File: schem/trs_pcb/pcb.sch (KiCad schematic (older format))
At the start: 10 parts, among them J101 2x3 female, J102 2x3 female, U101 74HCT245, U102 74HC165, U103 74HC595, U104 74HC595

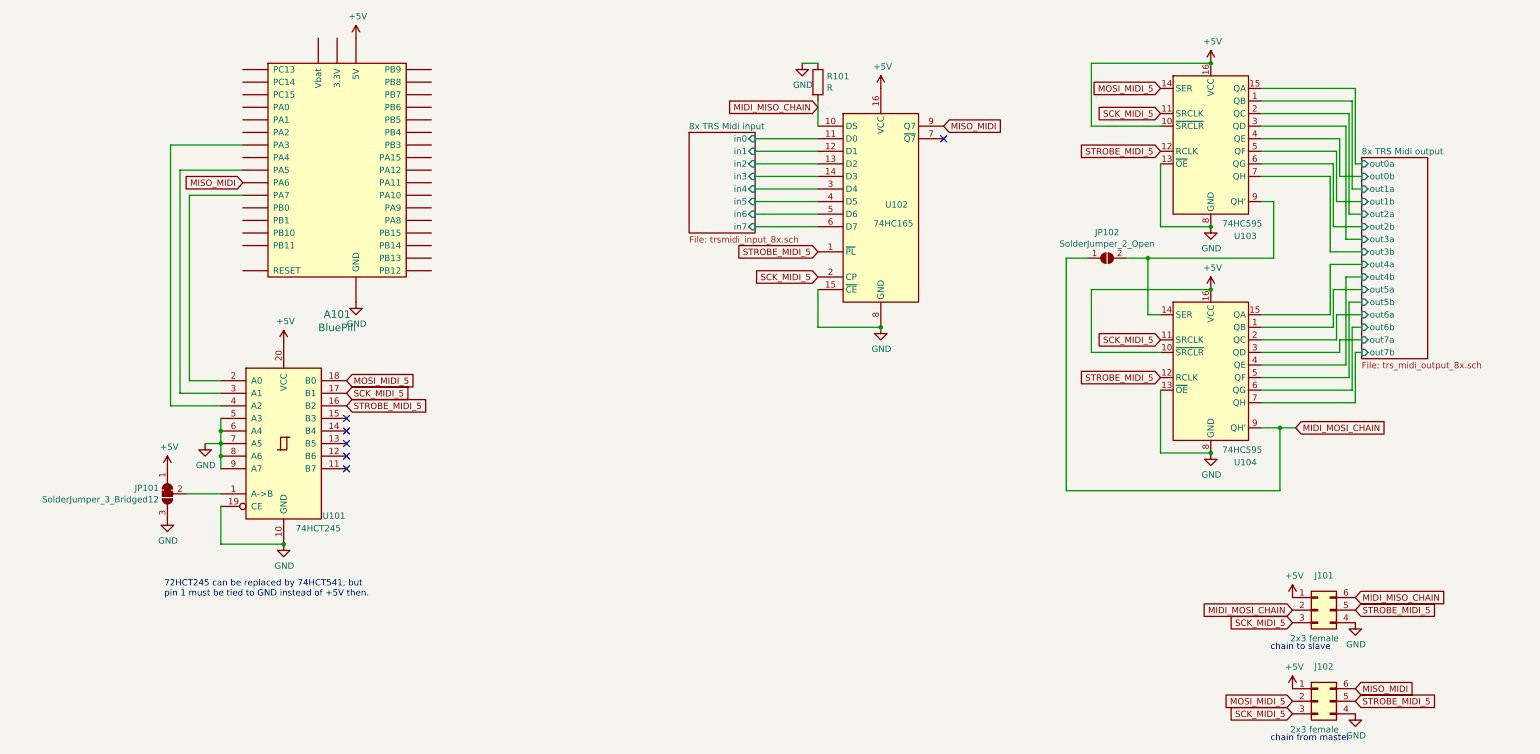
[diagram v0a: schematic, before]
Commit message: Come layout considerations
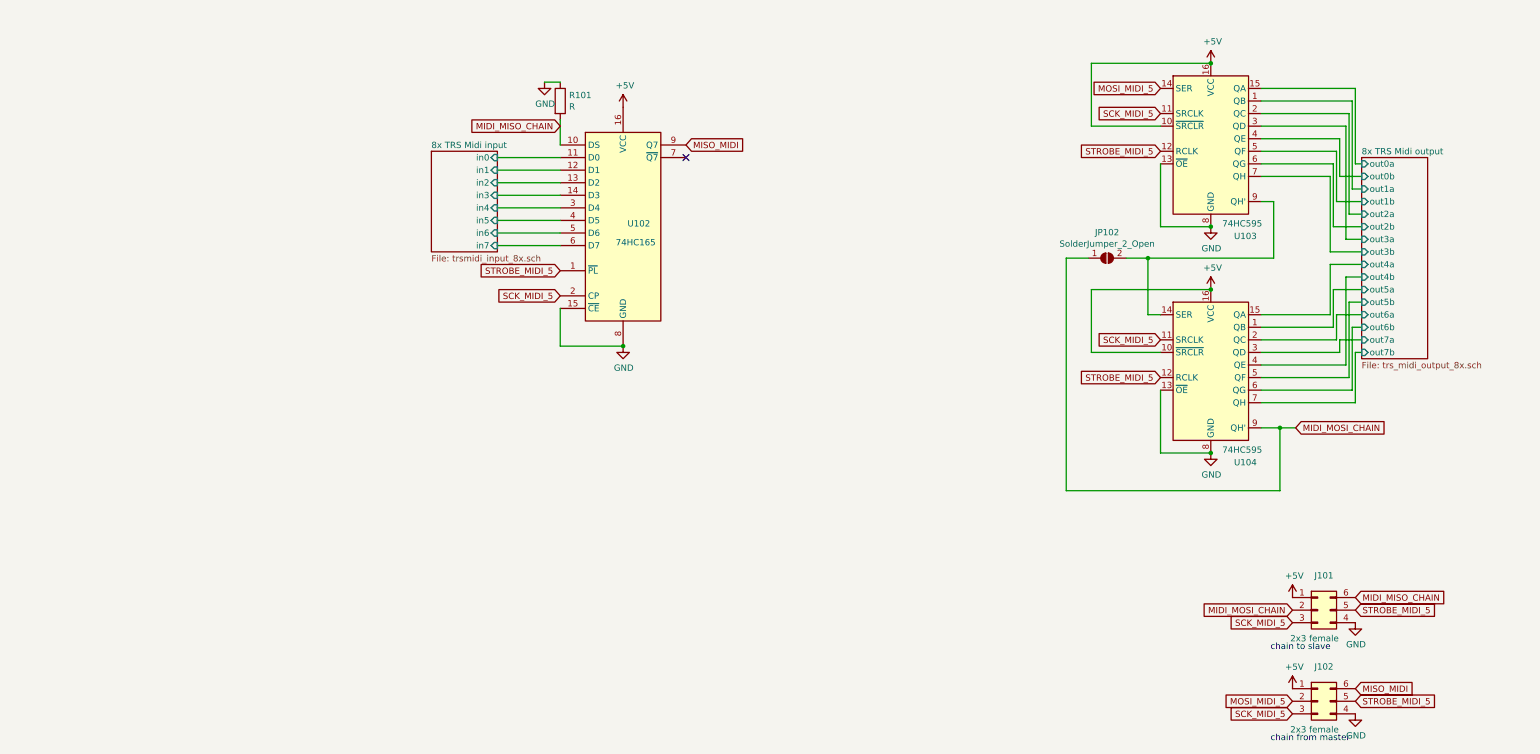
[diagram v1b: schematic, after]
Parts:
- removed A101: BluePill, footprints:BLUEPILL, symbol bluepill:BluePill
- removed JP101: SolderJumper_3_Bridged12, Jumper:SolderJumper-3_P2.0mm_Open_TrianglePad1.0x1.5mm, symbol Jumper:SolderJumper_3_Bridged12
- removed U101: 74HCT245, Package_DIP:DIP-20_W7.62mm, symbol 74xx:74HC245
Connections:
- no-connect marks 6 -> 1
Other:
- note removed: "72HCT245 can be replaced by 74HCT541, but\npin 1 must be tied to GND instead of +5V then."
- moved on the sheet: R101, U102
